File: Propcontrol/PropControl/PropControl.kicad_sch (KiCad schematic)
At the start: 80 parts, among them J1 Conn_01x08, J2 Conn_01x03_Pin, J3 Conn_01x05_Pin, J4 Conn_01x02_Pin, J5 Conn_01x02_Pin, Q1 CSD18533Q5A, Q2 CSD18533Q5A, Q3 CSD18533Q5A, Q4 CSD18533Q5A, Q5 CSD18533Q5A, Q6 CSD18533Q5A, U1 STM32F030F4P6, U2 UCC27301ADR, U4 UCC27301ADR, U5 TPS62933DRLR, U9 LM339D

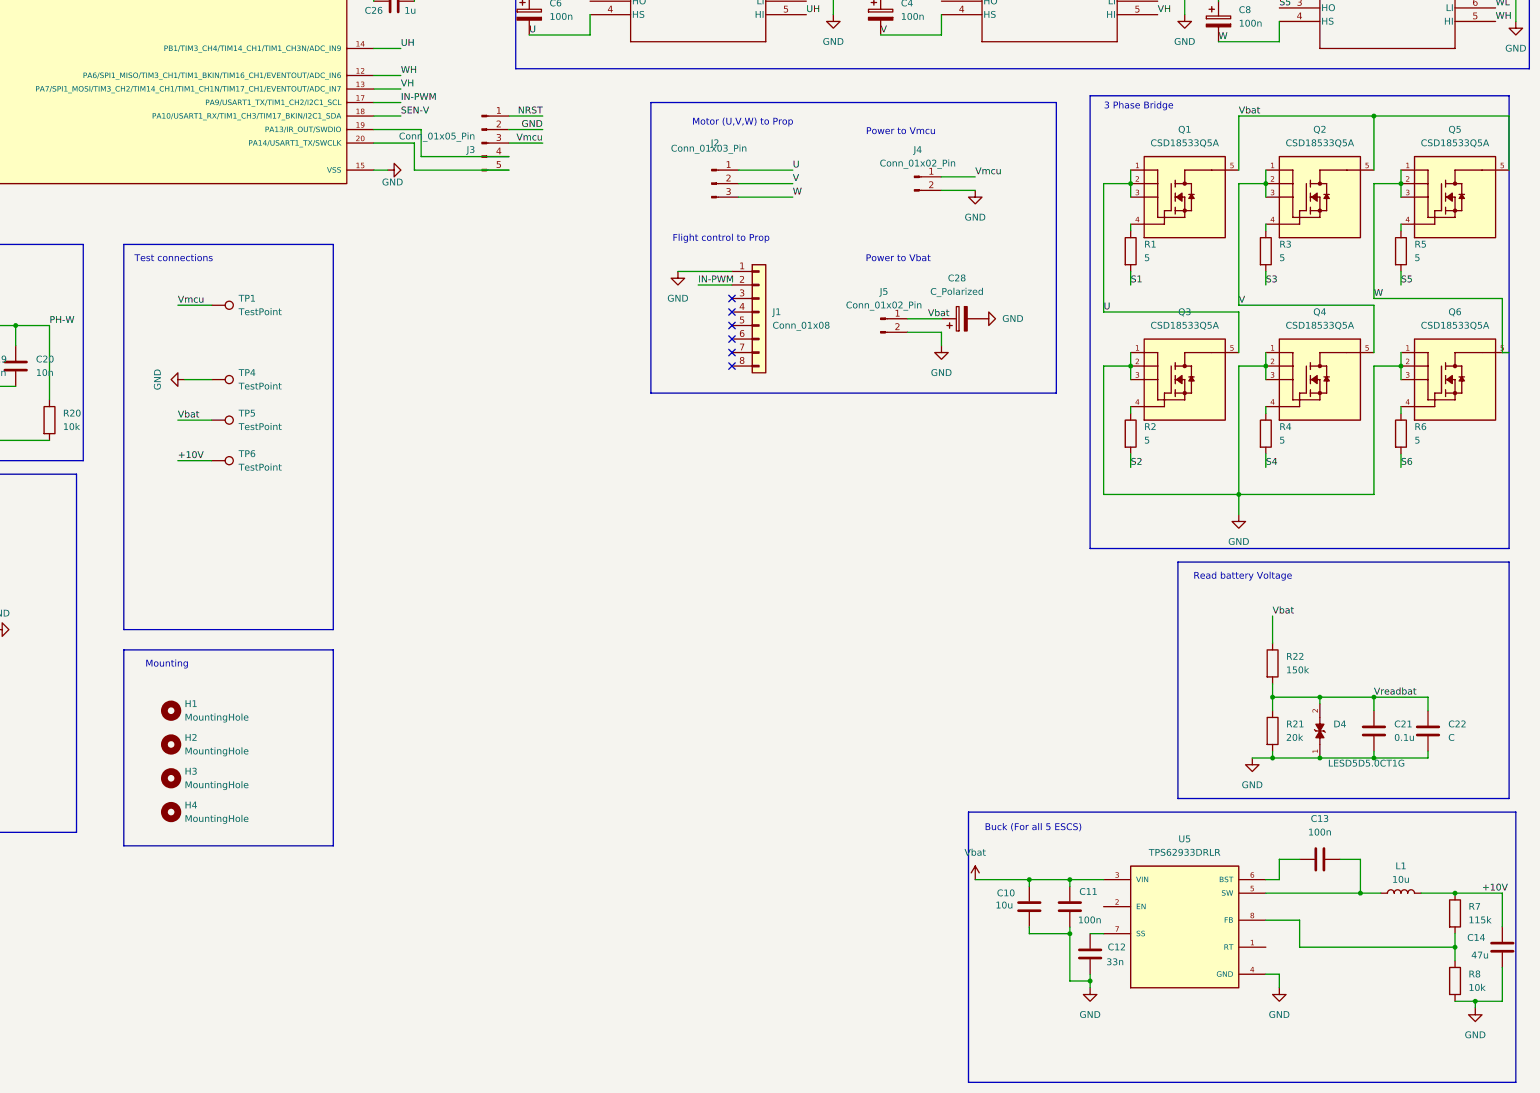
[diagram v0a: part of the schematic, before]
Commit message: changes january 29th
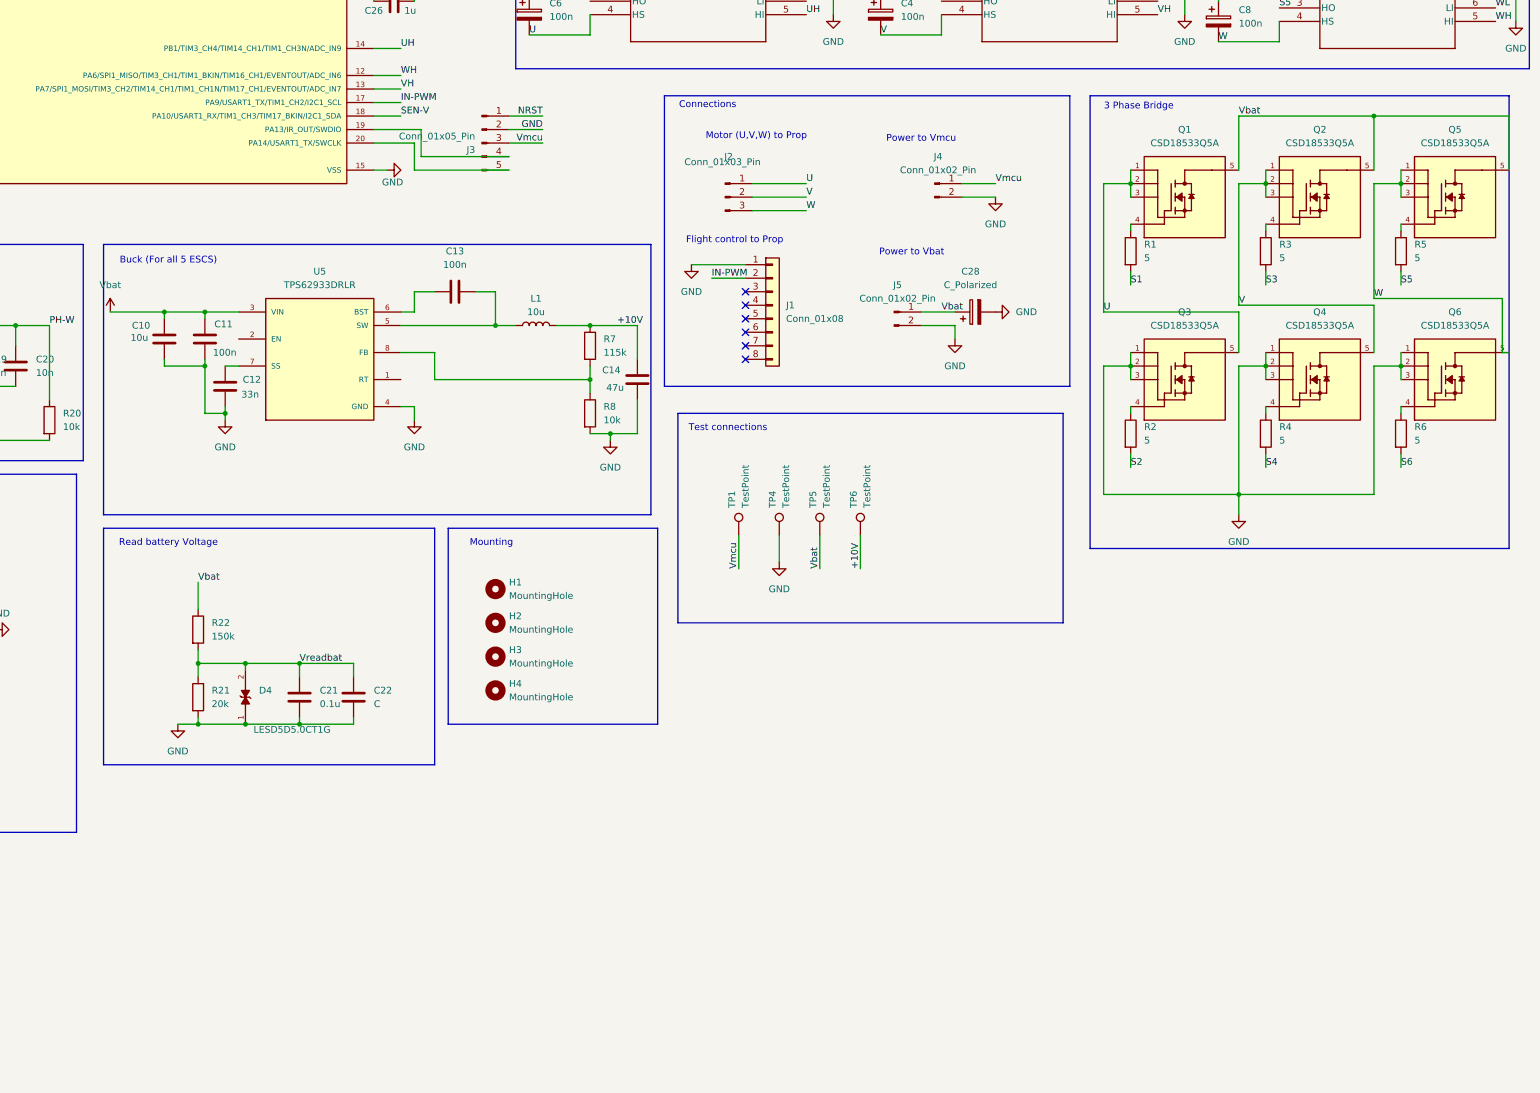
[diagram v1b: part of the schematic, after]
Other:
- note added: "Connections"
- moved on the sheet: C10, C11, C12, C13, C14, C21, C22, C28, D4, H1, H2, H3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
